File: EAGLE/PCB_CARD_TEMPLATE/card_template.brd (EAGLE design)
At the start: 24 x 60 mm, 8 parts, among them M1 MOUNTING_3M_3.2MM, X1 CONN_SMD_67P-P0.5-V_NASB0-S67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, X2 M.2_MKEY_FINGERS

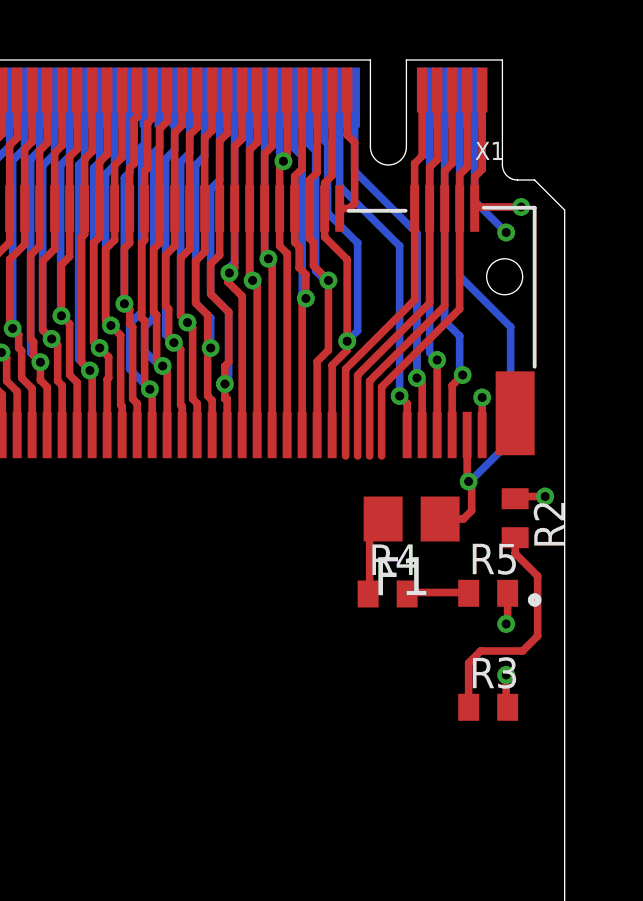
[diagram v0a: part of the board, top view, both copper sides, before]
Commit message: pic24 card is done, gerbers and jlc files generated
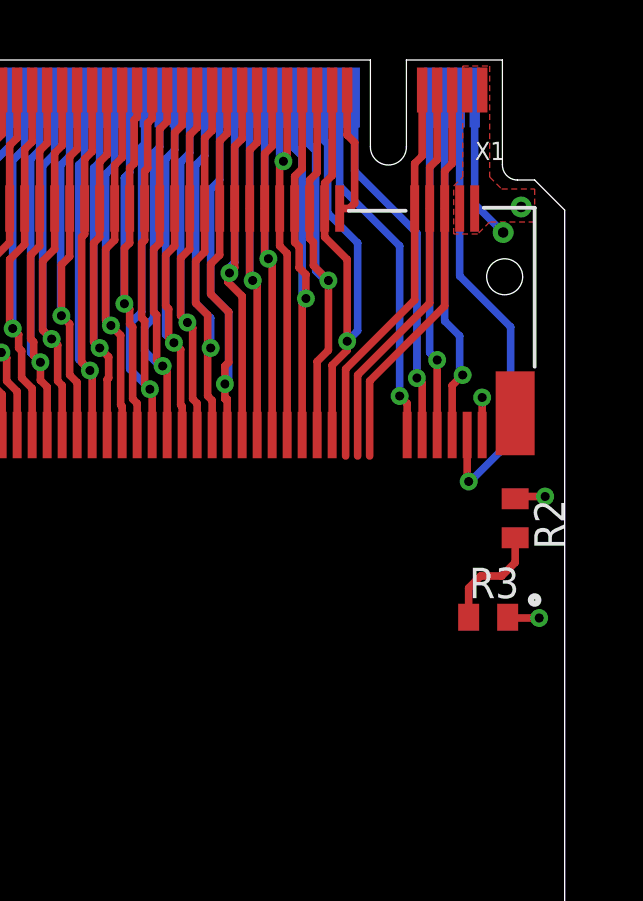
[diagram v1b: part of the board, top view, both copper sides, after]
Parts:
- removed F1: 100mA, _NIBE_rcl:R0805
- removed R4: 470R, _NIBE_rcl:R0603
- removed R5: LED_GREEN, _NIBE_rcl:R0603
- moved R3 3.00 mm to (21.4, 41.4)
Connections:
- removed net N$32: F1.1, X1.P$3, X2.72
- removed net N$35: X1.P$4, X2.73
- removed net N$40: R4.2, R5.1
- net +5V: now also X1.P$3, X2.72; no longer F1.2, R4.1
- net GND: now also X1.P$4, X2.73; no longer R5.2
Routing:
- net N$32: track 17.9 -> 0.00 mm, vias 1 -> 0
- net N$35: track 13.4 -> 0.00 mm
- net +5V: track 2.71 -> 15.7 mm, vias 0 -> 1
- net GND: track 15.5 -> 8.77 mm, vias 5 -> 4
- net N$33: track 7.73 -> 3.70 mm
- net N$40: track 2.11 -> 0.00 mm
- added copper zone on layer 1, net GND
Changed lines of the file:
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@@
 <attribute name="VALUE" x="2.5" y="54.25" locked="yes" size="0.6096" layer="27" font="vector" ratio="14"/>
-</element>
-<element name="F1" library="_NIBE_rcl" package="R0805" value="100mA" x="18.9" y="44.7" smashed="yes" rot="R180">
-<attribute name="NAME" x="19.535" y="43.43" size="1.27" layer="25" rot="R180"/>
-<attribute name="VALUE" x="19.535" y="47.24" size="1.27" layer="27" rot="R180"/>
 </element>
 <element name="R2" library="_NIBE_rcl" package="R0603" value="470R" x="22.35" y="44.725" smashed="yes" rot="R270">
@@
 <attribute name="VALUE" x="20.445" y="45.36" size="1.016" layer="27" rot="R270"/>
 </element>
-<element name="R3" library="_NIBE_rcl" package="R0603" value="LED_GREEN" x="21.45" y="38.425" smashed="yes">
-<attribute name="NAME" x="20.815" y="39.06" size="1.016" layer="25"/>
-<attribute name="VALUE" x="20.815" y="36.52" size="1.016" layer="27"/>
-</element>
-<element name="R4" library="_NIBE_rcl" package="R0603" value="470R" x="18.1" y="42.2" smashed="yes">
-<attribute name="NAME" x="17.465" y="42.835" size="1.016" layer="25"/>
-<attribute name="VALUE" x="17.465" y="40.295" size="1.016" layer="27"/>
-</element>
-<element name="R5" library="_NIBE_rcl" package="R0603" value="LED_GREEN" x="21.45" y="42.225" smashed="yes">
-<attribute name="NAME" x="20.815" y="42.86" size="1.016" layer="25"/>
-<attribute name="VALUE" x="20.815" y="40.32" size="1.016" layer="27"/>
+<element name="R3" library="_NIBE_rcl" package="R0603" value="LED_GREEN" x="21.45" y="41.425" smashed="yes">
+<attribute name="NAME" x="20.815" y="42.06" size="1.016" layer="25"/>
+<attribute name="VALUE" x="20.815" y="39.52" size="1.016" layer="27"/>
 </element>
 </elements>
@@
 <contactref element="X2" pad="75"/>
 <contactref element="R3" pad="2"/>
-<contactref element="R5" pad="2"/>
 <polygon width="0.254" layer="15" thermals="no">
 <vertex x="-1" y="-1"/>
@@
 </polygon>
 <via x="1.65" y="50.325" extent="1-16" drill="0.3"/>
-<via x="22.05" y="39.5" extent="1-16" drill="0.3"/>
-<via x="22.05" y="41.2" extent="1-16" drill="0.3"/>
-<wire x1="22.1" y1="42.225" x2="22.1" y2="41.25" width="0.254" layer="1"/>
-<wire x1="22.1" y1="41.25" x2="22.05" y2="41.2" width="0.254" layer="1"/>
-<wire x1="22.1" y1="38.425" x2="22.05" y2="38.475" width="0.254" layer="1"/>
-<wire x1="22.05" y1="38.475" x2="22.05" y2="39.5" width="0.254" layer="1"/>
-<via x="22.55" y="55.1" extent="1-16" drill="0.3"/>
-<wire x1="21" y1="55.049884375" x2="21.050115625" y2="55.1" width="0.254" layer="1"/>
-<wire x1="21.050115625" y1="55.1" x2="22.55" y2="55.1" width="0.254" layer="1"/>
-<wire x1="21.25" y1="56.35" x2="21.25" y2="59" width="0.254" layer="1"/>
-<wire x1="21" y1="55.049884375" x2="21" y2="56.1" width="0.254" layer="1"/>
-<wire x1="21" y1="56.1" x2="21.25" y2="56.35" width="0.254" layer="1"/>
+<via x="23.15" y="41.4" extent="1-16" drill="0.3"/>
+<wire x1="23.15" y1="41.4" x2="22.125" y2="41.4" width="0.254" layer="1"/>
+<wire x1="22.1" y1="41.425" x2="22.125" y2="41.4" width="0.254" layer="1"/>
+<via x="22.55" y="55.1" extent="1-16" drill="0.35"/>
 <wire x1="2.75" y1="59" x2="2.75" y2="58.15" width="0.254" layer="1"/>
 <wire x1="2.75" y1="58.15" x2="2.5" y2="57.9" width="0.254" layer="1"/>
@@
 <wire x1="2.6" y1="49.7" x2="1.975" y2="50.325" width="0.254" layer="1"/>
 <wire x1="1.975" y1="50.325" x2="1.65" y2="50.325" width="0.254" layer="1"/>
+<contactref element="X1" pad="P$4"/>
+<contactref element="X2" pad="73"/>
+<polygon width="0.1524" layer="1" thermals="no">
+<vertex x="20.3" y="54.2"/>
+<vertex x="20.3" y="55.8"/>
+<vertex x="20.6" y="56.1"/>
+<vertex x="20.6" y="59.8"/>
+<vertex x="21.5" y="59.8"/>
+<vertex x="21.5" y="56.1"/>
+<vertex x="21.9" y="55.7"/>
+<vertex x="23" y="55.7"/>
+<vertex x="23" y="54.6"/>
+<vertex x="21.5" y="54.6"/>
+<vertex x="21.1" y="54.2"/>
+</polygon>
+<wire x1="20.75" y1="59" x2="21.25" y2="59" width="0" layer="19" extent="1-1"/>
+<wire x1="21" y1="55.049884375" x2="21.25" y2="59" width="0" layer="19" extent="1-1"/>
+<wire x1="20.5" y1="55.049884375" x2="21" y2="55.049884375" width="0" layer="19" extent="1-1"/>
+<wire x1="22.55" y1="55.1" x2="21" y2="55.049884375" width="0" layer="19" extent="1-1"/>
+<wire x1="22.125" y1="41.4" x2="21" y2="55.049884375" width="0" layer="19" extent="1-1"/>
+<wire x1="2.75" y1="59" x2="20.75" y2="59" width="0" layer="19" extent="1-1"/>
+<wire x1="1.65" y1="50.325" x2="1.65" y2="55.3" width="0" layer="19" extent="1-1"/>
 </signal>
 <signal name="N$3">
@@
 <wire x1="20.5" y1="50.8" x2="20.5" y2="49.6" width="0.254" layer="16"/>
 </signal>
-<signal name="N$32">
-<contactref element="X1" pad="P$3"/>
-<contactref element="X2" pad="72"/>
-<contactref element="F1" pad="1"/>
-<wire x1="20.8" y1="45.95" x2="20.9" y2="45.85" width="0.254" layer="1"/>
-<wire x1="20.9" y1="45.85" x2="20.9" y2="44.975" width="0.254" layer="1"/>
-<wire x1="20.9" y1="44.975" x2="20.625" y2="44.7" width="0.254" layer="1"/>
-<wire x1="19.85" y1="44.7" x2="20.625" y2="44.7" width="0.254" layer="1"/>
-<wire x1="20.75" y1="47.499971875" x2="20.75" y2="46" width="0.254" layer="1"/>
-<wire x1="20.8" y1="45.95" x2="20.75" y2="46" width="0.254" layer="1"/>
-<via x="20.8" y="45.95" extent="1-16" drill="0.3"/>
-<wire x1="20.5" y1="52.8" x2="22.2" y2="51.1" width="0.254" layer="16"/>
-<wire x1="20.85" y1="45.95" x2="20.8" y2="45.95" width="0.254" layer="16"/>
-<wire x1="22.2" y1="51.1" x2="22.2" y2="47.3" width="0.254" layer="16"/>
-<wire x1="22.2" y1="47.3" x2="20.85" y2="45.95" width="0.254" layer="16"/>
-<wire x1="20.5" y1="52.8" x2="20.5" y2="58.75" width="0.254" layer="16"/>
-</signal>
-<signal name="N$35">
-<contactref element="X1" pad="P$4"/>
-<contactref element="X2" pad="73"/>
-<wire x1="20.75" y1="56.425" x2="20.75" y2="59" width="0.254" layer="1"/>
-<wire x1="20.5" y1="56.175" x2="20.75" y2="56.425" width="0.254" layer="1"/>
-<wire x1="20.5" y1="55.049884375" x2="20.5" y2="56.175" width="0.254" layer="1"/>
-<wire x1="20.5" y1="55.049884375" x2="20.5" y2="51.7" width="0.254" layer="1"/>
-<wire x1="20.5" y1="51.7" x2="17.9" y2="49.1" width="0.254" layer="1"/>
-<wire x1="17.9" y1="49.1" x2="17.9" y2="46.8" width="0.254" layer="1"/>
-</signal>
 <signal name="N$36">
 <contactref element="X1" pad="P$6"/>
@@
 <wire x1="22.35" y1="45.375" x2="22.425" y2="45.45" width="0.254" layer="1"/>
 <wire x1="22.425" y1="45.45" x2="23.35" y2="45.45" width="0.254" layer="1"/>
-<via x="22.05" y="54.25" extent="1-16" drill="0.3"/>
-<wire x1="21" y1="58.75" x2="21" y2="55.3" width="0.254" layer="16"/>
-<wire x1="22.05" y1="54.25" x2="21" y2="55.3" width="0.254" layer="16"/>
+<via x="21.95" y="54.25" extent="1-16" drill="0.35"/>
+<wire x1="21" y1="58.75" x2="21" y2="55.2" width="0.254" layer="16"/>
+<wire x1="21.95" y1="54.25" x2="21" y2="55.2" width="0.254" layer="16"/>
 </signal>
 <signal name="+5V">
-<contactref element="F1" pad="2"/>
-<contactref element="R4" pad="1"/>
-<wire x1="17.5" y1="44.25" x2="17.5" y2="42.25" width="0.254" layer="1"/>
-<wire x1="17.95" y1="44.7" x2="17.5" y2="44.25" width="0.254" layer="1"/>
-<wire x1="17.5" y1="42.25" x2="17.45" y2="42.2" width="0.254" layer="1"/>
+<contactref element="X1" pad="P$3"/>
+<contactref element="X2" pad="72"/>
+<wire x1="20.75" y1="47.499971875" x2="20.75" y2="46" width="0.254" layer="1"/>
+<wire x1="20.8" y1="45.95" x2="20.75" y2="46" width="0.254" layer="1"/>
+<via x="20.8" y="45.95" extent="1-16" drill="0.3"/>
+<wire x1="20.5" y1="52.8" x2="22.2" y2="51.1" width="0.254" layer="16"/>
+<wire x1="20.85" y1="45.95" x2="20.8" y2="45.95" width="0.254" layer="16"/>
+<wire x1="22.2" y1="51.1" x2="22.2" y2="47.3" width="0.254" layer="16"/>
+<wire x1="22.2" y1="47.3" x2="20.85" y2="45.95" width="0.254" layer="16"/>
+<wire x1="20.5" y1="52.8" x2="20.5" y2="58.75" width="0.254" layer="16"/>
 </signal>
 <signal name="N$33">
 <contactref element="R2" pad="2"/>
 <contactref element="R3" pad="1"/>
-<wire x1="20.8" y1="38.425" x2="20.8" y2="39.9" width="0.254" layer="1"/>
-<wire x1="22.35" y1="43.55" x2="22.35" y2="44.075" width="0.254" layer="1"/>
-<wire x1="20.8" y1="39.9" x2="21.2" y2="40.3" width="0.254" layer="1"/>
-<wire x1="21.2" y1="40.3" x2="22.6" y2="40.3" width="0.254" layer="1"/>
-<wire x1="22.6" y1="40.3" x2="23.1" y2="40.8" width="0.254" layer="1"/>
-<wire x1="23.1" y1="40.8" x2="23.1" y2="42.8" width="0.254" layer="1"/>
-<wire x1="23.1" y1="42.8" x2="22.35" y2="43.55" width="0.254" layer="1"/>
-</signal>
-<signal name="N$40">
-<contactref element="R5" pad="1"/>
-<contactref element="R4" pad="2"/>
-<wire x1="20.75" y1="42.25" x2="18.75" y2="42.25" width="0.254" layer="1"/>
-<wire x1="18.75" y1="42.25" x2="18.75" y2="42.2" width="0.254" layer="1"/>
-<wire x1="20.75" y1="42.25" x2="20.8" y2="42.225" width="0.254" layer="1"/>
+<wire x1="22.35" y1="44.075" x2="22.35" y2="43.25" width="0.254" layer="1"/>
+<wire x1="21.9" y1="42.8" x2="21.2" y2="42.8" width="0.254" layer="1"/>
+<wire x1="21.2" y1="42.8" x2="20.8" y2="42.4" width="0.254" layer="1"/>
+<wire x1="20.8" y1="42.4" x2="20.8" y2="41.425" width="0.254" layer="1"/>
+<wire x1="22.35" y1="43.25" x2="21.9" y2="42.8" width="0.254" layer="1"/>
 </signal>
 </signals>
